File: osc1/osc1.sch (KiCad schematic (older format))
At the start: 61 parts

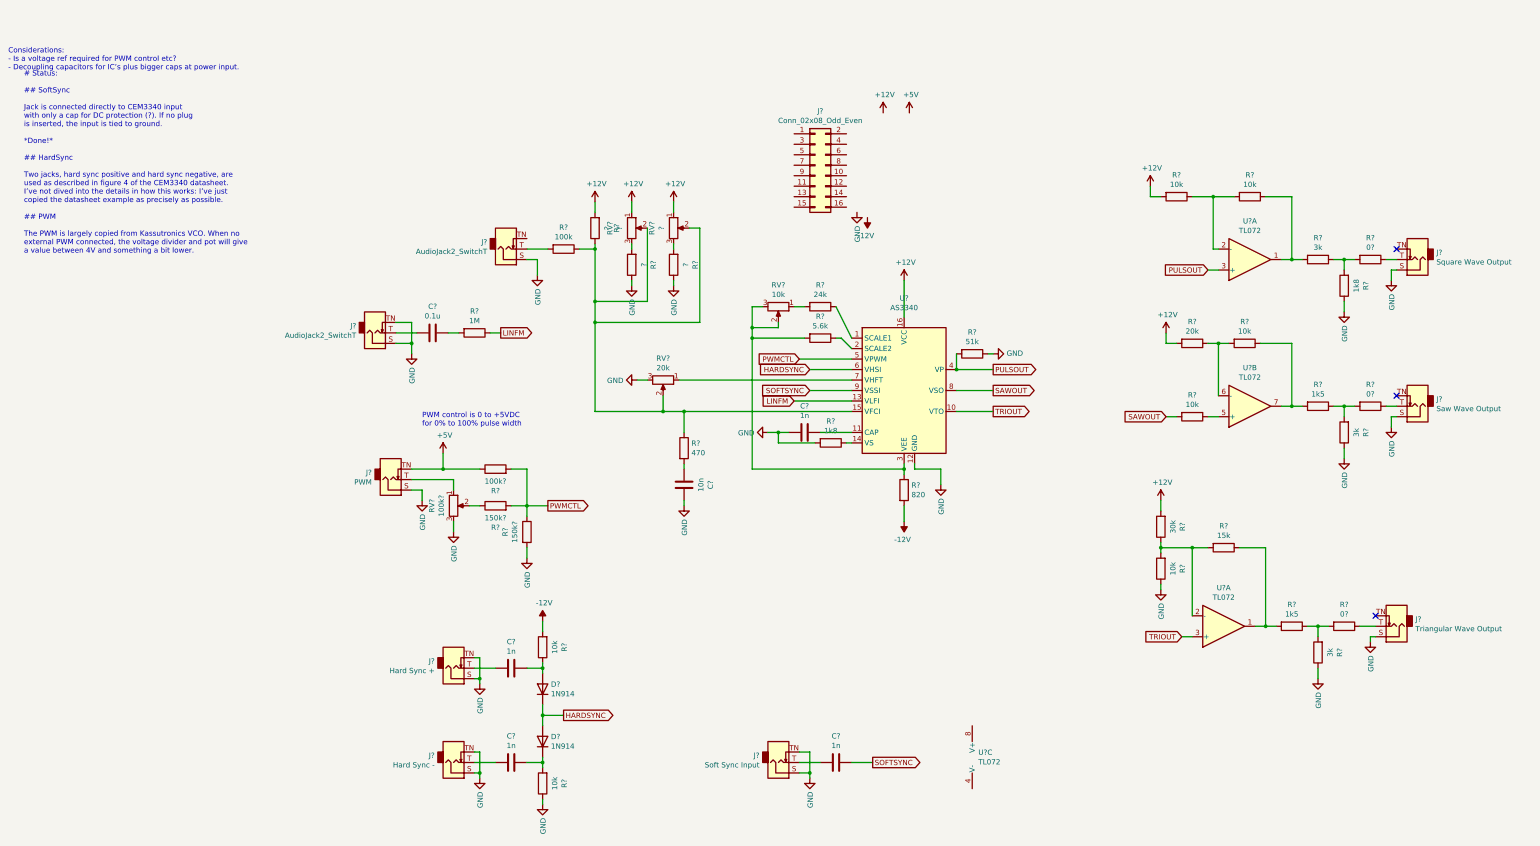
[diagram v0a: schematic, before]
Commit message: Revert "PWM"
This reverts commit d376f1211e99f4c40a807b6edc23770ccc192675.

This is to solve a merge conflict. The changes in "PWM" will applied
again.
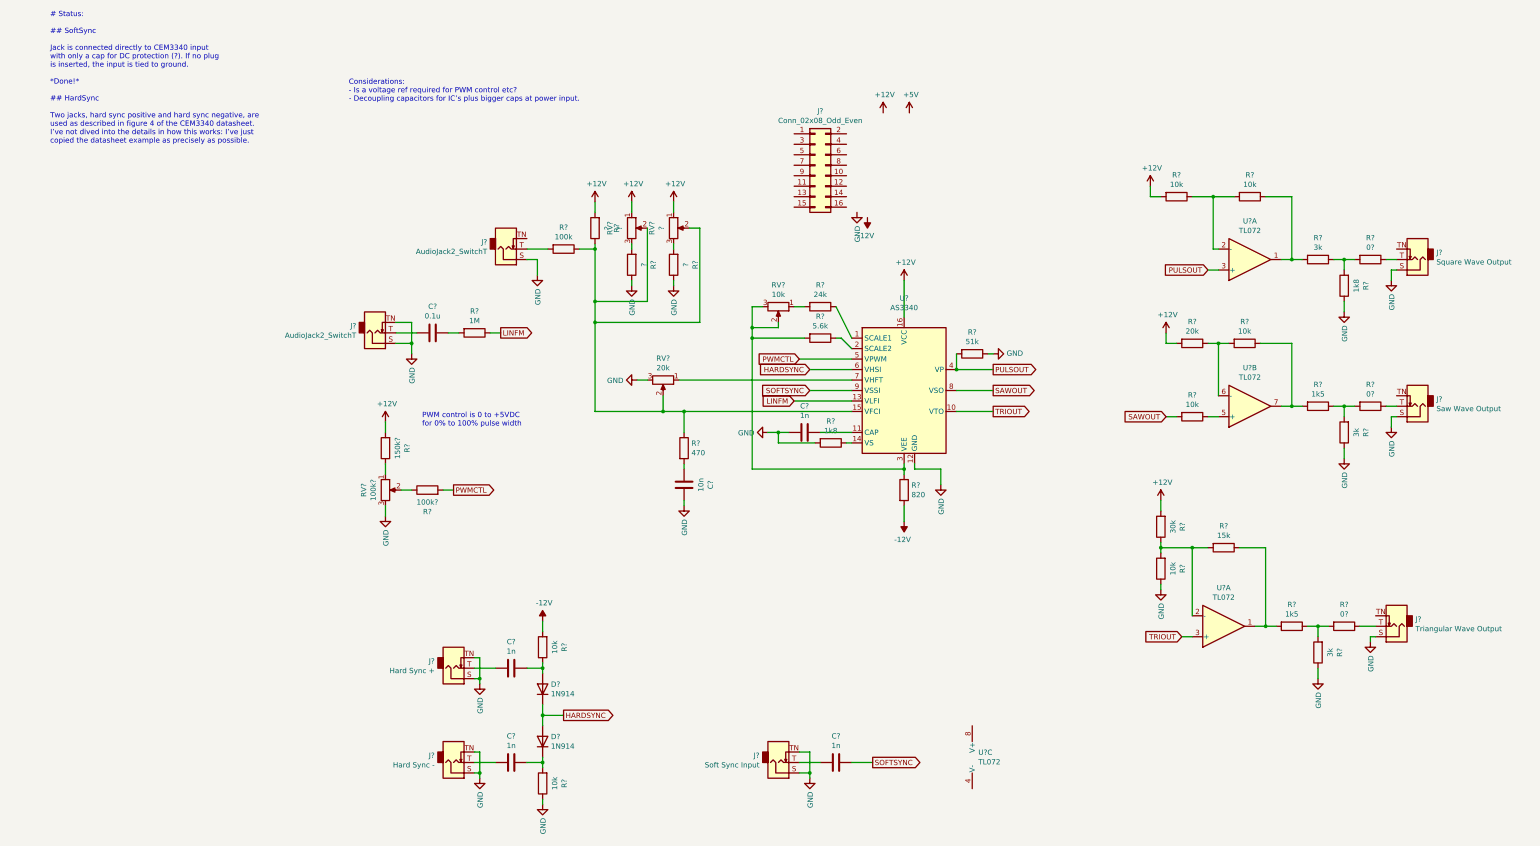
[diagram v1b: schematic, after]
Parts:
- removed J?: PWM, symbol Connector:AudioJack2_SwitchT
- removed R?: 150k?, symbol Device:R
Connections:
- net +12V: now also R?.2
- net +5V: no longer R?.1
- net PWMCTL: no longer R?.2
- net at RV?.1: now also R?.1
- net at RV?.2: now also R?.1; no longer R?.1
- no-connect marks 3 -> 0
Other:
- moved on the sheet: R?, RV?
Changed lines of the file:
@@
 EESchema Schematic File Version 4
+LIBS:osc1-cache
 EELAYER 30 0
 EELAYER END
@@
 L Device:R_POT RV?
 U 1 1 5DCC115F
-P 1500 4600
-F 0 "RV?" V 1293 4600 50  0000 C CNN
-F 1 "100k?" V 1384 4600 50  0000 C CNN
-F 2 "" H 1500 4600 50  0001 C CNN
-F 3 "~" H 1500 4600 50  0001 C CNN
-	1    1500 4600
+P 850 4450
+F 0 "RV?" V 643 4450 50  0000 C CNN
+F 1 "100k?" V 734 4450 50  0000 C CNN
+F 2 "" H 850 4450 50  0001 C CNN
+F 3 "~" H 850 4450 50  0001 C CNN
+	1    850  4450
+	1    0    0    -1
+$EndComp
+$Comp
+L power:+12V #PWR?
+U 1 1 5DCCB73D
+P 850 3800
+F 0 "#PWR?" H 850 3650 50  0001 C CNN
+F 1 "+12V" H 865 3973 50  0000 C CNN
+F 2 "" H 850 3800 50  0001 C CNN
+F 3 "" H 850 3800 50  0001 C CNN
+	1    850  3800
 	1    0    0    -1
 $EndComp
@@
 L Device:R R?
 U 1 1 5DCCC2FE
-P 1900 4600
-F 0 "R?" V 1693 4600 50  0000 C CNN
-F 1 "150k?" V 1784 4600 50  0000 C CNN
-F 2 "" V 1830 4600 50  0001 C CNN
-F 3 "~" H 1900 4600 50  0001 C CNN
-	1    1900 4600
+P 850 4050
+F 0 "R?" V 643 4050 50  0000 C CNN
+F 1 "150k?" V 734 4050 50  0000 C CNN
+F 2 "" V 780 4050 50  0001 C CNN
+F 3 "~" H 850 4050 50  0001 C CNN
+	1    850  4050
+	-1   0    0    1
+$EndComp
+Wire Wire Line
+	850  3900 850  3800
+Wire Wire Line
+	850  4200 850  4300
+$Comp
+L power:GND #PWR?
+U 1 1 5DCD529A
+P 850 4700
+F 0 "#PWR?" H 850 4450 50  0001 C CNN
+F 1 "GND" V 855 4572 50  0000 R CNN
+F 2 "" H 850 4700 50  0001 C CNN
+F 3 "" H 850 4700 50  0001 C CNN
+	1    850  4700
+	1    0    0    -1
+$EndComp
+Wire Wire Line
+	850  4700 850  4600
+$Comp
+L Device:R R?
+U 1 1 5DCD9BD4
+P 1250 4450
+F 0 "R?" V 1043 4450 50  0000 C CNN
+F 1 "100k?" V 1134 4450 50  0000 C CNN
+F 2 "" V 1180 4450 50  0001 C CNN
+F 3 "~" H 1250 4450 50  0001 C CNN
+	1    1250 4450
 	0    -1   -1   0
 $EndComp
-$Comp
-L Device:R R?
-U 1 1 5DCD9BD4
-P 1900 4250
-F 0 "R?" V 1693 4250 50  0000 C CNN
-F 1 "100k?" V 1784 4250 50  0000 C CNN
-F 2 "" V 1830 4250 50  0001 C CNN
-F 3 "~" H 1900 4250 50  0001 C CNN
-	1    1900 4250
-	0    -1   -1   0
-$EndComp
-Text GLabel 2400 4600 2    50   Output ~ 0
+Wire Wire Line
+	1000 4450 1100 4450
+Wire Wire Line
+	1400 4450 1500 4450
+Text GLabel 1500 4450 2    50   Output ~ 0
 PWMCTL
 Text Notes 1200 3850 0    50   ~ 0
 PWM control is 0 to +5VDC\nfor 0% to 100% pulse width
-Text Notes -2750 450  0    50   ~ 0
+Text Notes 500  750  0    50   ~ 0
 Considerations:\n- Is a voltage ref required for PWM control etc?\n- Decoupling capacitors for IC’s plus bigger caps at power input.
 $Comp
@@
 	4900 6950 4900 7150
 Connection ~ 4900 7150
-Text Notes -2600 2200 0    50   ~ 0
-# Status:\n\n## SoftSync\n\nJack is connected directly to CEM3340 input\nwith only a cap for DC protection (?). If no plug\nis inserted, the input is tied to ground.\n\n*Done!*\n\n## HardSync\n\nTwo jacks, hard sync positive and hard sync negative, are\nused as described in figure 4 of the CEM3340 datasheet.\nI’ve not dived into the details in how this works: I’ve just\ncopied the datasheet example as precisely as possible.\n\n## PWM\n\nThe PWM is largely copied from Kassutronics VCO. When no\nexternal PWM connected, the voltage divider and pot will give\na value between 4V and something a bit lower.
+Text Notes -2350 1150 0    50   ~ 0
+# Status:\n\n## SoftSync\n\nJack is connected directly to CEM3340 input\nwith only a cap for DC protection (?). If no plug\nis inserted, the input is tied to ground.\n\n*Done!*\n\n## HardSync\n\nTwo jacks, hard sync positive and hard sync negative, are\nused as described in figure 4 of the CEM3340 datasheet.\nI’ve not dived into the details in how this works: I’ve just\ncopied the datasheet example as precisely as possible.
 Wire Wire Line
 	1700 6050 1750 6050
@@
 	1100 2850 1100 3050
 Connection ~ 1100 3050
-$Comp
-L Connector:AudioJack2_SwitchT J?
-U 1 1 5E2872A3
-P 900 4350
-F 0 "J?" H 720 4283 50  0000 R CNN
-F 1 "PWM" H 720 4374 50  0000 R CNN
-F 2 "" H 900 4350 50  0001 C CNN
-F 3 "~" H 900 4350 50  0001 C CNN
-	1    900  4350
-	1    0    0    1
-$EndComp
-NoConn ~ 10500 3550
-NoConn ~ 10500 2150
-NoConn ~ 10300 5650
-$Comp
-L power:+5V #PWR?
-U 1 1 5E2D8E2C
-P 1400 4100
-F 0 "#PWR?" H 1400 3950 50  0001 C CNN
-F 1 "+5V" H 1415 4273 50  0000 C CNN
-F 2 "" H 1400 4100 50  0001 C CNN
-F 3 "" H 1400 4100 50  0001 C CNN
-	1    1400 4100
-	1    0    0    -1
-$EndComp
-Wire Wire Line
-	1400 4250 1400 4100
-Wire Wire Line
-	1100 4250 1400 4250
-Connection ~ 1400 4250
-$Comp
-L power:GND #PWR?
-U 1 1 5E321467
-P 1200 4550
-F 0 "#PWR?" H 1200 4300 50  0001 C CNN
-F 1 "GND" V 1205 4422 50  0000 R CNN
-F 2 "" H 1200 4550 50  0001 C CNN
-F 3 "" H 1200 4550 50  0001 C CNN
-	1    1200 4550
-	1    0    0    -1
-$EndComp
-Wire Wire Line
-	1200 4550 1200 4450
-Wire Wire Line
-	1200 4450 1100 4450
-$Comp
-L power:GND #PWR?
-U 1 1 5E32EAD1
-P 1500 4850
-F 0 "#PWR?" H 1500 4600 50  0001 C CNN
-F 1 "GND" V 1505 4722 50  0000 R CNN
-F 2 "" H 1500 4850 50  0001 C CNN
-F 3 "" H 1500 4850 50  0001 C CNN
-	1    1500 4850
-	1    0    0    -1
-$EndComp
-Wire Wire Line
-	1500 4750 1500 4850
-Wire Wire Line
-	1500 4350 1500 4450
-Wire Wire Line
-	1100 4350 1500 4350
-Wire Wire Line
-	1650 4600 1750 4600
-Wire Wire Line
-	1400 4250 1750 4250
-Wire Wire Line
-	2050 4600 2200 4600
-Wire Wire Line
-	2200 4600 2200 4250
-Wire Wire Line
-	2200 4250 2050 4250
-$Comp
-L Device:R R?
-U 1 1 5E392C21
-P 2200 4850
-F 0 "R?" V 1993 4850 50  0000 C CNN
-F 1 "150k?" V 2084 4850 50  0000 C CNN
-F 2 "" V 2130 4850 50  0001 C CNN
-F 3 "~" H 2200 4850 50  0001 C CNN
-	1    2200 4850
-	1    0    0    -1
-$EndComp
-Wire Wire Line
-	2200 4700 2200 4600
-Connection ~ 2200 4600
-$Comp
-L power:GND #PWR?
-U 1 1 5E39B988
-P 2200 5100
-F 0 "#PWR?" H 2200 4850 50  0001 C CNN
-F 1 "GND" V 2205 4972 50  0000 R CNN
-F 2 "" H 2200 5100 50  0001 C CNN
-F 3 "" H 2200 5100 50  0001 C CNN
-	1    2200 5100
-	1    0    0    -1
-$EndComp
-Wire Wire Line
-	2200 5100 2200 5000
-Wire Wire Line
-	2200 4600 2400 4600
 $EndSCHEMATC

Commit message: PWM
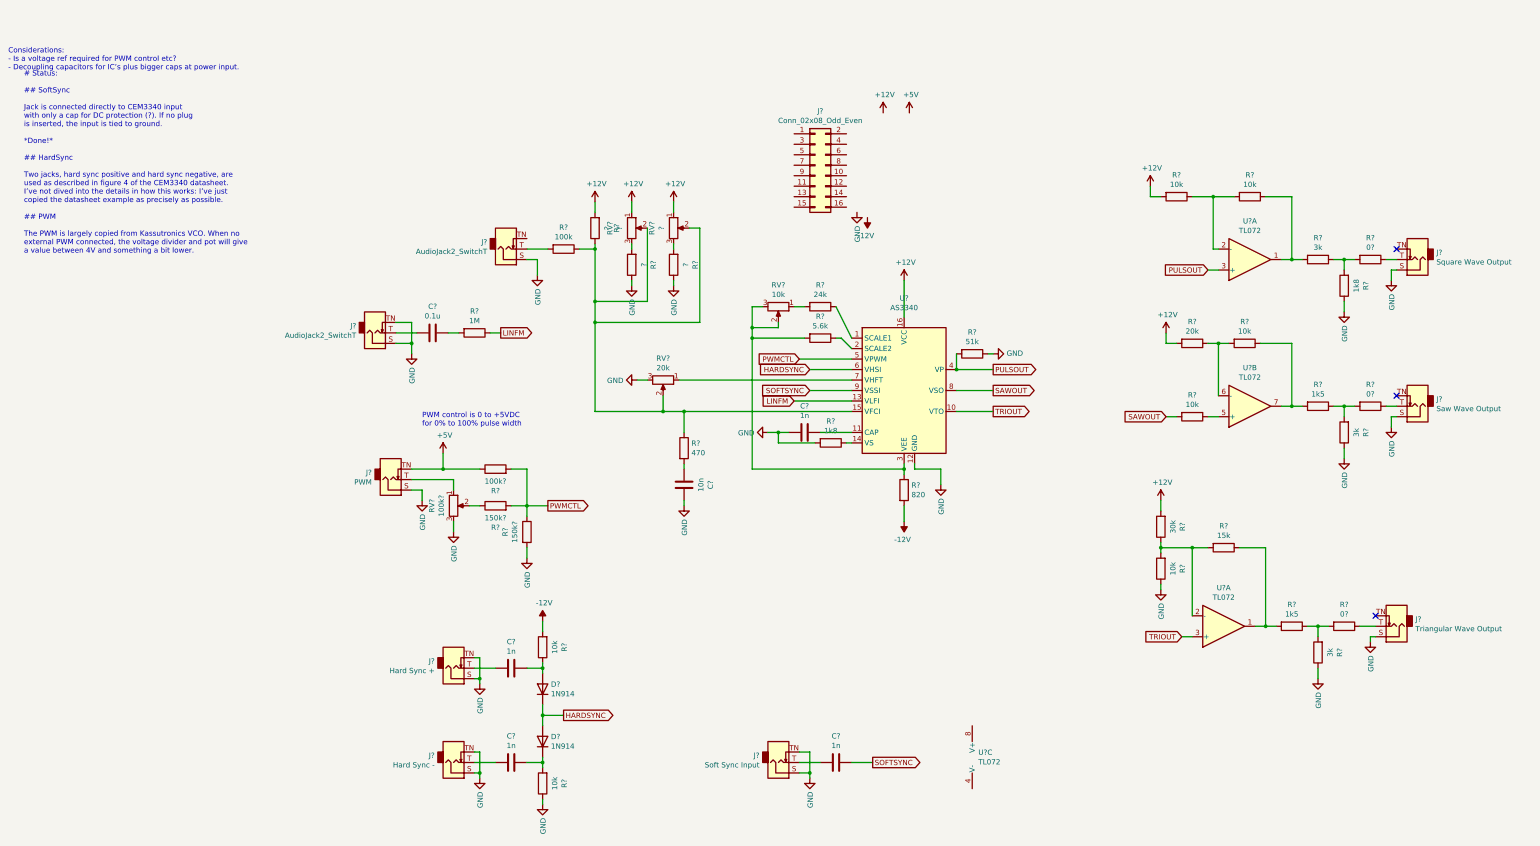
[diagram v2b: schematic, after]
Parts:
- added J?: PWM, symbol Connector:AudioJack2_SwitchT
- added R?: 150k?, symbol Device:R
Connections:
- net +12V: no longer R?.2
- net +5V: now also R?.1, J?.TN
- net GND: now also J?.S, R?.2
- net PWMCTL: now also R?.2, R?.1
- net at RV?.1: now also J?.T; no longer R?.1
- net at RV?.2: now also R?.1; no longer R?.1
- no-connect marks 0 -> 3
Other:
- moved on the sheet: R?, RV?
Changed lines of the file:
@@
 EESchema Schematic File Version 4
-LIBS:osc1-cache
 EELAYER 30 0
 EELAYER END
@@
 L Device:R_POT RV?
 U 1 1 5DCC115F
-P 850 4450
-F 0 "RV?" V 643 4450 50  0000 C CNN
-F 1 "100k?" V 734 4450 50  0000 C CNN
-F 2 "" H 850 4450 50  0001 C CNN
-F 3 "~" H 850 4450 50  0001 C CNN
-	1    850  4450
-	1    0    0    -1
-$EndComp
-$Comp
-L power:+12V #PWR?
-U 1 1 5DCCB73D
-P 850 3800
-F 0 "#PWR?" H 850 3650 50  0001 C CNN
-F 1 "+12V" H 865 3973 50  0000 C CNN
-F 2 "" H 850 3800 50  0001 C CNN
-F 3 "" H 850 3800 50  0001 C CNN
-	1    850  3800
+P 1500 4600
+F 0 "RV?" V 1293 4600 50  0000 C CNN
+F 1 "100k?" V 1384 4600 50  0000 C CNN
+F 2 "" H 1500 4600 50  0001 C CNN
+F 3 "~" H 1500 4600 50  0001 C CNN
+	1    1500 4600
 	1    0    0    -1
 $EndComp
@@
 L Device:R R?
 U 1 1 5DCCC2FE
-P 850 4050
-F 0 "R?" V 643 4050 50  0000 C CNN
-F 1 "150k?" V 734 4050 50  0000 C CNN
-F 2 "" V 780 4050 50  0001 C CNN
-F 3 "~" H 850 4050 50  0001 C CNN
-	1    850  4050
-	-1   0    0    1
-$EndComp
-Wire Wire Line
-	850  3900 850  3800
-Wire Wire Line
-	850  4200 850  4300
-$Comp
-L power:GND #PWR?
-U 1 1 5DCD529A
-P 850 4700
-F 0 "#PWR?" H 850 4450 50  0001 C CNN
-F 1 "GND" V 855 4572 50  0000 R CNN
-F 2 "" H 850 4700 50  0001 C CNN
-F 3 "" H 850 4700 50  0001 C CNN
-	1    850  4700
-	1    0    0    -1
-$EndComp
-Wire Wire Line
-	850  4700 850  4600
+P 1900 4600
+F 0 "R?" V 1693 4600 50  0000 C CNN
+F 1 "150k?" V 1784 4600 50  0000 C CNN
+F 2 "" V 1830 4600 50  0001 C CNN
+F 3 "~" H 1900 4600 50  0001 C CNN
+	1    1900 4600
+	0    -1   -1   0
+$EndComp
 $Comp
 L Device:R R?
 U 1 1 5DCD9BD4
-P 1250 4450
-F 0 "R?" V 1043 4450 50  0000 C CNN
-F 1 "100k?" V 1134 4450 50  0000 C CNN
-F 2 "" V 1180 4450 50  0001 C CNN
-F 3 "~" H 1250 4450 50  0001 C CNN
-	1    1250 4450
+P 1900 4250
+F 0 "R?" V 1693 4250 50  0000 C CNN
+F 1 "100k?" V 1784 4250 50  0000 C CNN
+F 2 "" V 1830 4250 50  0001 C CNN
+F 3 "~" H 1900 4250 50  0001 C CNN
+	1    1900 4250
 	0    -1   -1   0
 $EndComp
-Wire Wire Line
-	1000 4450 1100 4450
-Wire Wire Line
-	1400 4450 1500 4450
-Text GLabel 1500 4450 2    50   Output ~ 0
+Text GLabel 2400 4600 2    50   Output ~ 0
 PWMCTL
 Text Notes 1200 3850 0    50   ~ 0
 PWM control is 0 to +5VDC\nfor 0% to 100% pulse width
-Text Notes 500  750  0    50   ~ 0
+Text Notes -2750 450  0    50   ~ 0
 Considerations:\n- Is a voltage ref required for PWM control etc?\n- Decoupling capacitors for IC’s plus bigger caps at power input.
 $Comp
@@
 	4900 6950 4900 7150
 Connection ~ 4900 7150
-Text Notes -2350 1150 0    50   ~ 0
-# Status:\n\n## SoftSync\n\nJack is connected directly to CEM3340 input\nwith only a cap for DC protection (?). If no plug\nis inserted, the input is tied to ground.\n\n*Done!*\n\n## HardSync\n\nTwo jacks, hard sync positive and hard sync negative, are\nused as described in figure 4 of the CEM3340 datasheet.\nI’ve not dived into the details in how this works: I’ve just\ncopied the datasheet example as precisely as possible.
+Text Notes -2600 2200 0    50   ~ 0
+# Status:\n\n## SoftSync\n\nJack is connected directly to CEM3340 input\nwith only a cap for DC protection (?). If no plug\nis inserted, the input is tied to ground.\n\n*Done!*\n\n## HardSync\n\nTwo jacks, hard sync positive and hard sync negative, are\nused as described in figure 4 of the CEM3340 datasheet.\nI’ve not dived into the details in how this works: I’ve just\ncopied the datasheet example as precisely as possible.\n\n## PWM\n\nThe PWM is largely copied from Kassutronics VCO. When no\nexternal PWM connected, the voltage divider and pot will give\na value between 4V and something a bit lower.
 Wire Wire Line
 	1700 6050 1750 6050
@@
 	1100 2850 1100 3050
 Connection ~ 1100 3050
+$Comp
+L Connector:AudioJack2_SwitchT J?
+U 1 1 5E2872A3
+P 900 4350
+F 0 "J?" H 720 4283 50  0000 R CNN
+F 1 "PWM" H 720 4374 50  0000 R CNN
+F 2 "" H 900 4350 50  0001 C CNN
+F 3 "~" H 900 4350 50  0001 C CNN
+	1    900  4350
+	1    0    0    1
+$EndComp
+NoConn ~ 10500 3550
+NoConn ~ 10500 2150
+NoConn ~ 10300 5650
+$Comp
+L power:+5V #PWR?
+U 1 1 5E2D8E2C
+P 1400 4100
+F 0 "#PWR?" H 1400 3950 50  0001 C CNN
+F 1 "+5V" H 1415 4273 50  0000 C CNN
+F 2 "" H 1400 4100 50  0001 C CNN
+F 3 "" H 1400 4100 50  0001 C CNN
+	1    1400 4100
+	1    0    0    -1
+$EndComp
+Wire Wire Line
+	1400 4250 1400 4100
+Wire Wire Line
+	1100 4250 1400 4250
+Connection ~ 1400 4250
+$Comp
+L power:GND #PWR?
+U 1 1 5E321467
+P 1200 4550
+F 0 "#PWR?" H 1200 4300 50  0001 C CNN
+F 1 "GND" V 1205 4422 50  0000 R CNN
+F 2 "" H 1200 4550 50  0001 C CNN
+F 3 "" H 1200 4550 50  0001 C CNN
+	1    1200 4550
+	1    0    0    -1
+$EndComp
+Wire Wire Line
+	1200 4550 1200 4450
+Wire Wire Line
+	1200 4450 1100 4450
+$Comp
+L power:GND #PWR?
+U 1 1 5E32EAD1
+P 1500 4850
+F 0 "#PWR?" H 1500 4600 50  0001 C CNN
+F 1 "GND" V 1505 4722 50  0000 R CNN
+F 2 "" H 1500 4850 50  0001 C CNN
+F 3 "" H 1500 4850 50  0001 C CNN
+	1    1500 4850
+	1    0    0    -1
+$EndComp
+Wire Wire Line
+	1500 4750 1500 4850
+Wire Wire Line
+	1500 4350 1500 4450
+Wire Wire Line
+	1100 4350 1500 4350
+Wire Wire Line
+	1650 4600 1750 4600
+Wire Wire Line
+	1400 4250 1750 4250
+Wire Wire Line
+	2050 4600 2200 4600
+Wire Wire Line
+	2200 4600 2200 4250
+Wire Wire Line
+	2200 4250 2050 4250
+$Comp
+L Device:R R?
+U 1 1 5E392C21
+P 2200 4850
+F 0 "R?" V 1993 4850 50  0000 C CNN
+F 1 "150k?" V 2084 4850 50  0000 C CNN
+F 2 "" V 2130 4850 50  0001 C CNN
+F 3 "~" H 2200 4850 50  0001 C CNN
+	1    2200 4850
+	1    0    0    -1
+$EndComp
+Wire Wire Line
+	2200 4700 2200 4600
+Connection ~ 2200 4600
+$Comp
+L power:GND #PWR?
+U 1 1 5E39B988
+P 2200 5100
+F 0 "#PWR?" H 2200 4850 50  0001 C CNN
+F 1 "GND" V 2205 4972 50  0000 R CNN
+F 2 "" H 2200 5100 50  0001 C CNN
+F 3 "" H 2200 5100 50  0001 C CNN
+	1    2200 5100
+	1    0    0    -1
+$EndComp
+Wire Wire Line
+	2200 5100 2200 5000
+Wire Wire Line
+	2200 4600 2400 4600
 $EndSCHEMATC
